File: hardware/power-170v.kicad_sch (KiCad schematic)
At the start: 2 parts

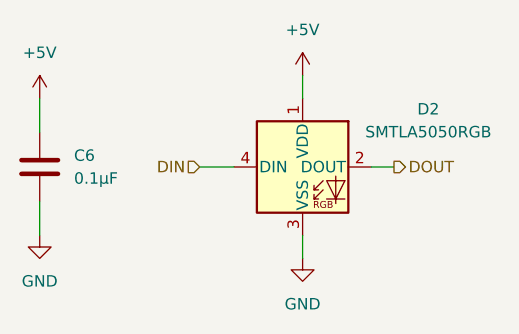
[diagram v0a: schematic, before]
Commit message: Progress point
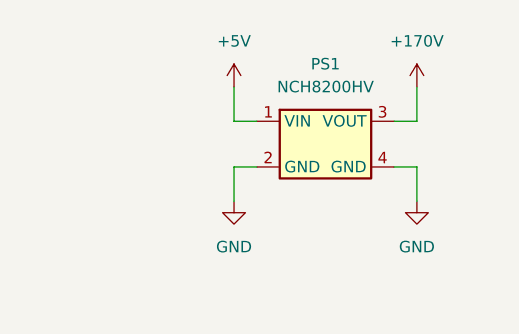
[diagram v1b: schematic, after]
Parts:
- removed C6: 0.1µF, Capacitor_SMD:C_0805_2012Metric, symbol Device:C
- removed D2: SMTLA5050RGB, LED_SMD:LED_WS2812B_PLCC4_5.0x5.0mm_P3.2mm, symbol LED:WS2812B
- added PS1: NCH8200HV, nch8200hv:NCH8200HV, symbol nch8200hv:NCH8200HV
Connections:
- net +5V: now also PS1.1 (VIN)
- net GND: now also PS1.2 (GND), PS1.4 (GND)
- new net +170V: PS1.3 (VOUT)
